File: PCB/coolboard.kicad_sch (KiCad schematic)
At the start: 35 parts, among them J1 USB_C_Receptacle_USB2.0_14P, J2 Conn_01x20, J3 Conn_01x20, J4 Conn_01x03, SW1 SW_Push, U1 RP2040, U2 MCP1700x-330xxTT, U4 W25Q16JVUXIQ TR, Y1 12MHz

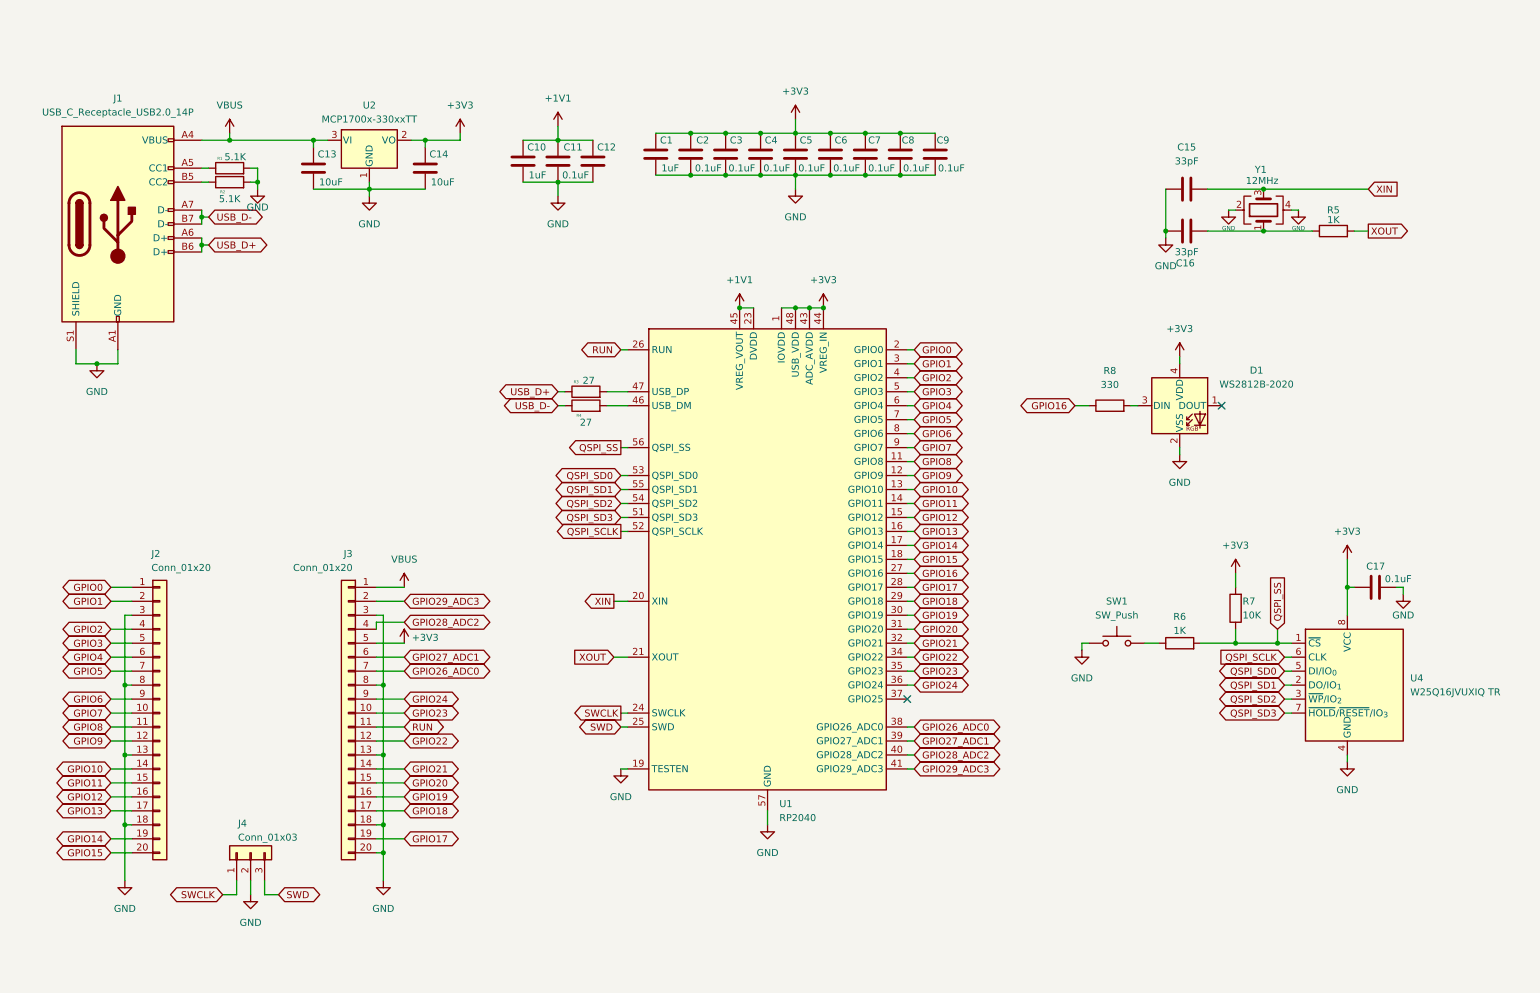
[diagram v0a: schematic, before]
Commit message: Update production zip file with latest changes
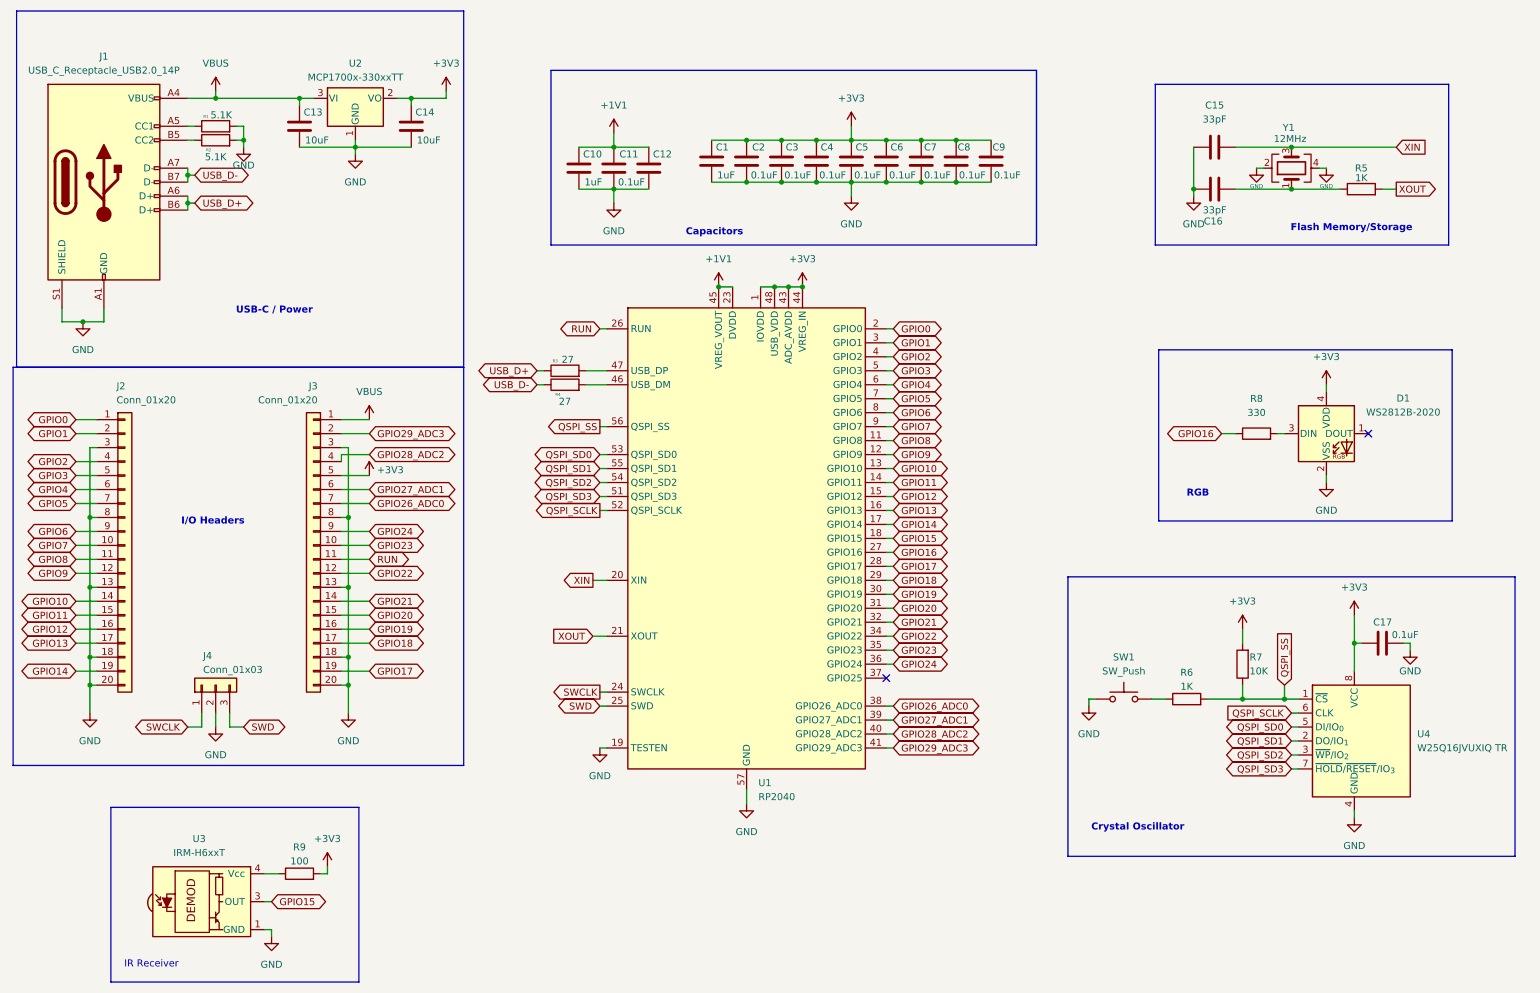
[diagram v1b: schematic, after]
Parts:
- added R9: 100, Capacitor_SMD:C_0402_1005Metric, symbol Device:R
- added U3: IRM-H6xxT, OptoDevice:Everlight_IRM-H6xxT, symbol Interface_Optical:IRM-H6xxT
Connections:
- net +3V3: now also R9.2
- net GND: now also J2.20 (Pin_20), U3.1 (GND), U3.2 (GND)
- net GPIO15: now also U3.3 (OUT); no longer J2.20 (Pin_20)
- new net: R9.1, U3.4 (Vcc)
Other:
- note added: "Capacitors"
- note added: "Crystal Oscillator"
- note added: "Flash Memory/Storage"
- note added: "I/O Headers"
- note added: "IR Receiver"
- note added: "RGB"
- note added: "USB-C / Power"
- moved on the sheet: C1, C10, C11, C12, C13, C14, C15, C16, C17, C2, C3, C4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
